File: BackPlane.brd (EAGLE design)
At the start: 134.6 x 116.5 mm, 1 part

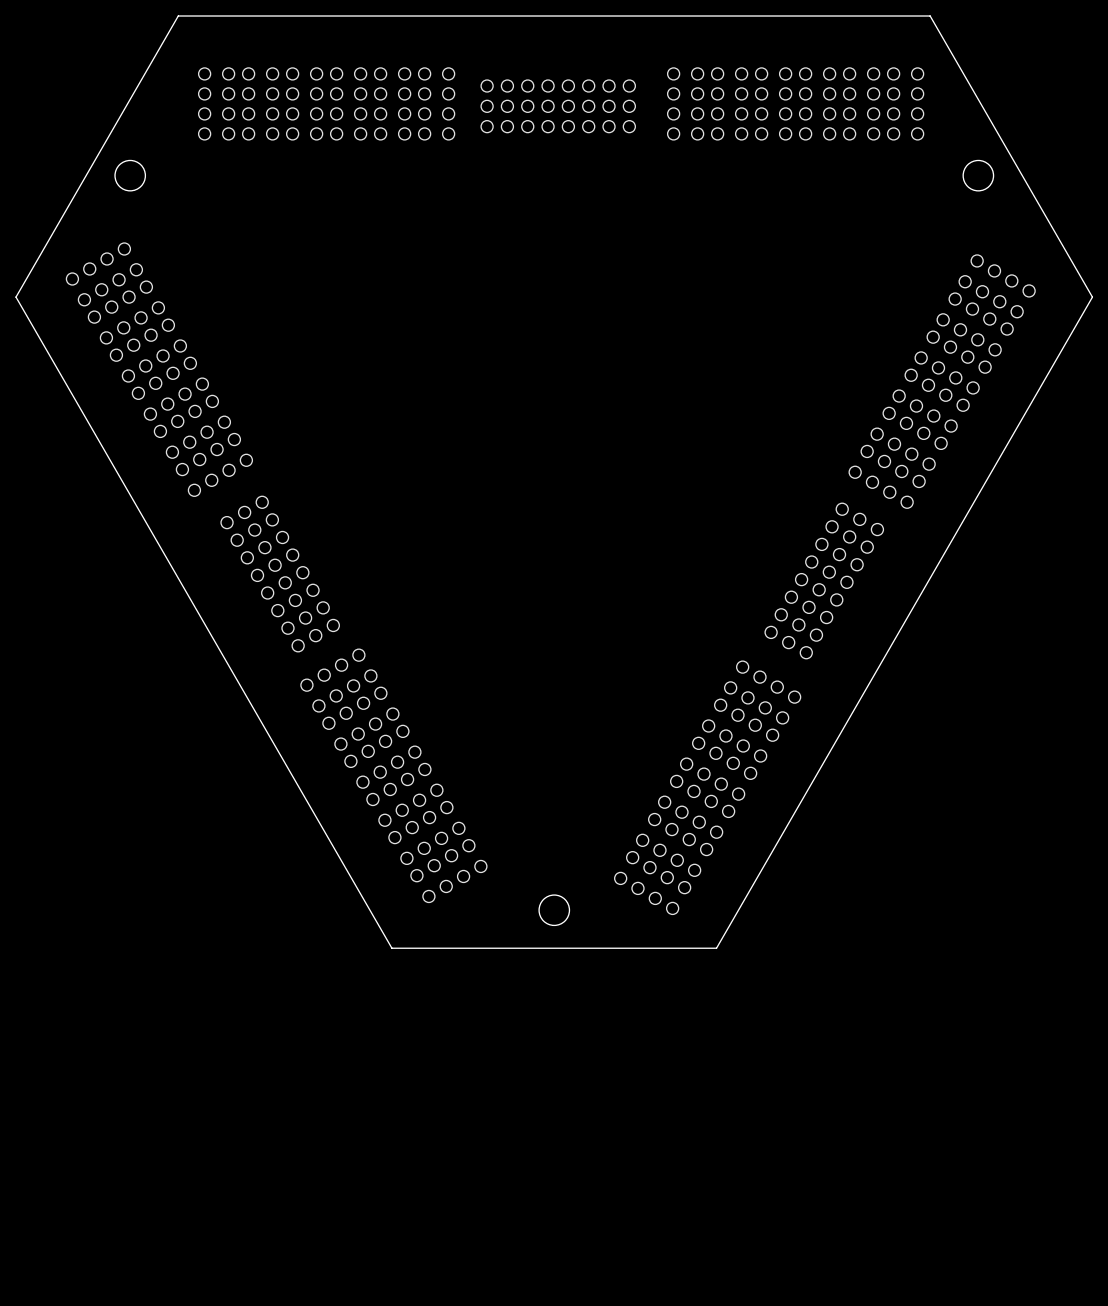
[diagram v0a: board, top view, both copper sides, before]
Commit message: progress
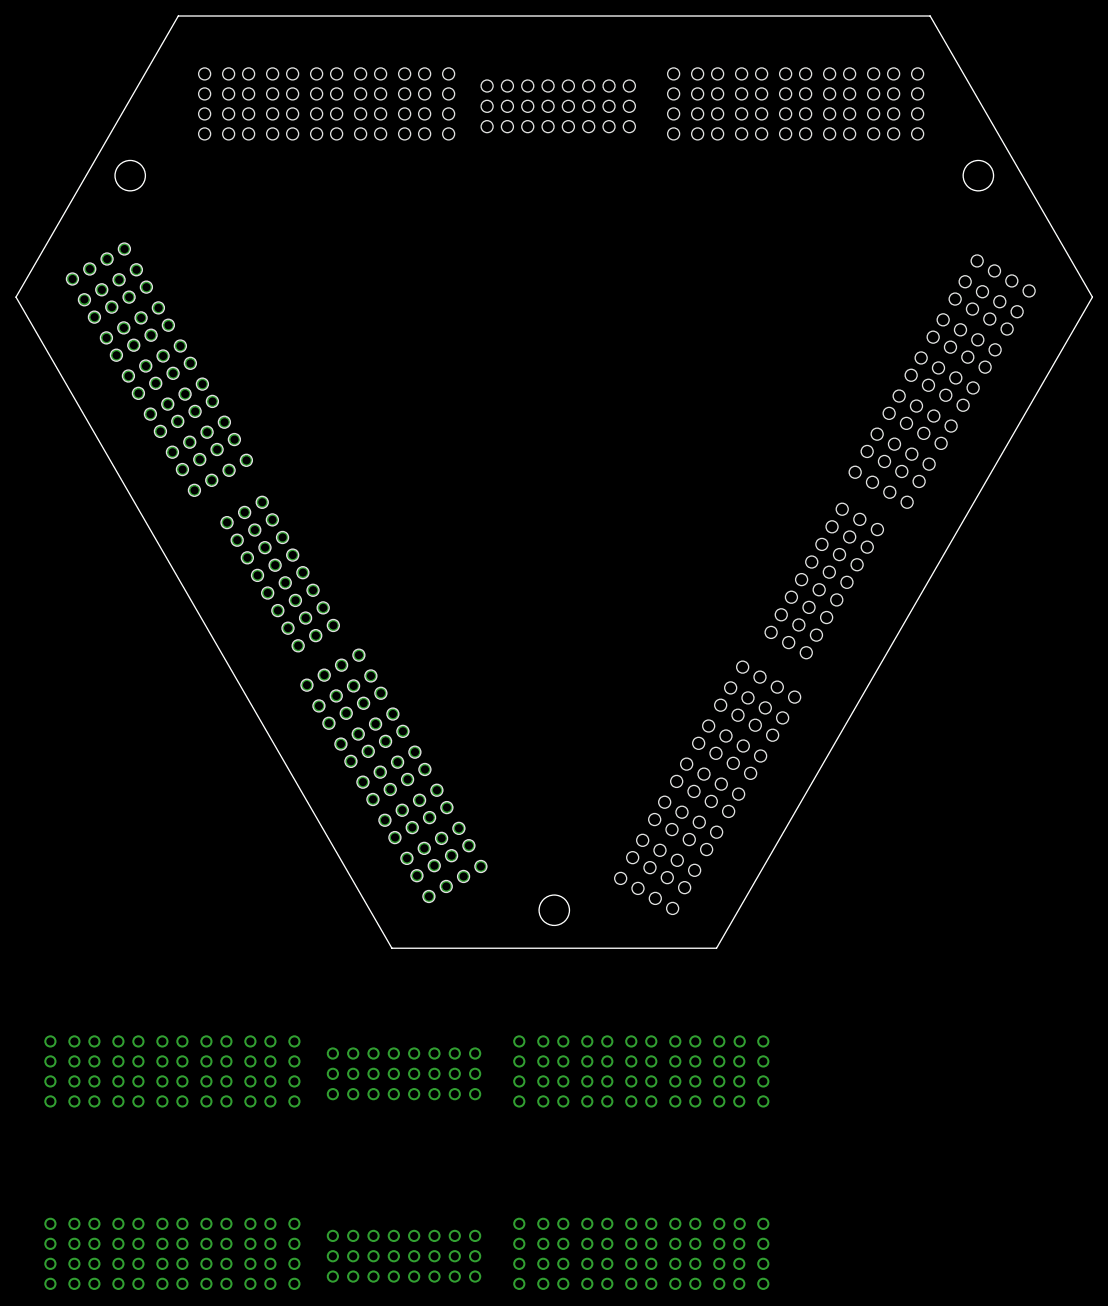
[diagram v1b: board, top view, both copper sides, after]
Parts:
- added U$2, U$3, U$4: THICC_CONNECTOR, THICC_CONNECTOR:THICC_CONNECTOR
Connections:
- new net +12V: U$2.15, U$2.16, U$2.23, U$2.24, U$3.15, U$3.16, U$3.23, U$3.24, U$4.15, U$4.16, U$4.23, U$4.24
- new net +12V_GND: U$2.13, U$2.14, U$2.21, U$2.22, U$3.13, U$3.14, U$3.21, U$3.22, U$4.13, U$4.14, U$4.21, U$4.22
- new net +5V: U$2.11, U$2.12, U$2.19, U$2.20, U$3.11, U$3.12, U$3.19, U$3.20, U$4.11, U$4.12, U$4.19, U$4.20
- new net +5V_GND: U$2.10, U$2.17, U$2.18, U$2.9, U$3.10, U$3.17, U$3.18, U$3.9, U$4.10, U$4.17, U$4.18, U$4.9
- new net B1: U$2.P1-13, U$2.P1-14, U$2.P1-15, U$2.P1-16, U$2.P2-17, U$2.P2-18, U$2.P2-19, U$2.P2-20, U$4.P1-13, U$4.P1-14, U$4.P1-15, U$4.P1-16, U$4.P2-17, U$4.P2-18, U$4.P2-19, U$4.P2-20
- new net B2: U$2.P2-1, U$2.P2-2, U$2.P2-3, U$2.P2-4, U$2.P2-5, U$2.P2-6, U$2.P2-7, U$2.P2-8, U$4.P2-1, U$4.P2-2, U$4.P2-3, U$4.P2-4, U$4.P2-5, U$4.P2-6, U$4.P2-7, U$4.P2-8
- new net B3: U$2.P3-25, U$2.P3-26, U$2.P3-27, U$2.P3-28, U$2.P4-5, U$2.P4-6, U$2.P4-7, U$2.P4-8, U$3.P3-25, U$3.P3-26, U$3.P3-27, U$3.P3-28, U$3.P4-5, U$3.P4-6, U$3.P4-7, U$3.P4-8, U$4.P3-25, U$4.P3-26, U$4.P3-27, U$4.P3-28, U$4.P4-5, U$4.P4-6, U$4.P4-7, U$4.P4-8
- new net B4: U$2.P3-13, U$2.P3-14, U$2.P3-15, U$2.P3-16, U$2.P4-10, U$2.P4-11, U$2.P4-12, U$2.P4-9, U$3.P3-13, U$3.P3-14, U$3.P3-15, U$3.P3-16, U$3.P4-10, U$3.P4-11, U$3.P4-12, U$3.P4-9, U$4.P3-13, U$4.P3-14, U$4.P3-15, U$4.P3-16, U$4.P4-10, U$4.P4-11, U$4.P4-12, U$4.P4-9
- new net B5: U$3.P1-13, U$3.P1-14, U$3.P1-15, U$3.P1-16, U$3.P2-17, U$3.P2-18, U$3.P2-19, U$3.P2-20
- new net B6: U$3.P2-1, U$3.P2-2, U$3.P2-3, U$3.P2-4, U$3.P2-5, U$3.P2-6, U$3.P2-7, U$3.P2-8
- new net CAN_H: U$2.8, U$3.8, U$4.8
- new net CAN_L: U$2.7, U$3.7, U$4.7
- new net R1: U$2.P1-1, U$2.P1-2, U$2.P1-21, U$2.P1-22, U$2.P1-23, U$2.P1-24, U$2.P1-3, U$2.P1-4, U$4.P1-1, U$4.P1-2, U$4.P1-21, U$4.P1-22, U$4.P1-23, U$4.P1-24, U$4.P1-3, U$4.P1-4
- new net R2: U$2.P1-10, U$2.P1-11, U$2.P1-12, U$2.P1-9, U$2.P2-13, U$2.P2-14, U$2.P2-15, U$2.P2-16, U$4.P1-10, U$4.P1-11, U$4.P1-12, U$4.P1-9, U$4.P2-13, U$4.P2-14, U$4.P2-15, U$4.P2-16
- new net R3: U$2.P3-17, U$2.P3-18, U$2.P3-19, U$2.P3-20, U$2.P4-13, U$2.P4-14, U$2.P4-15, U$2.P4-16, U$3.P3-17, U$3.P3-18, U$3.P3-19, U$3.P3-20, U$4.P3-17, U$4.P3-18, U$4.P3-19, U$4.P3-20, U$4.P4-13, U$4.P4-14, U$4.P4-15, U$4.P4-16
- new net R4: U$2.P3-1, U$2.P3-2, U$2.P3-3, U$2.P3-4, U$2.P3-5, U$2.P3-6, U$2.P3-7, U$2.P3-8, U$3.P3-1, U$3.P3-2, U$3.P3-3, U$3.P3-4, U$3.P3-5, U$3.P3-6, U$3.P3-7, U$3.P3-8, U$4.P3-1, U$4.P3-2, U$4.P3-3, U$4.P3-4, U$4.P3-5, U$4.P3-6, U$4.P3-7, U$4.P3-8
- new net R5: U$3.P1-1, U$3.P1-2, U$3.P1-21, U$3.P1-22, U$3.P1-23, U$3.P1-24, U$3.P1-3, U$3.P1-4
- new net R6: U$3.P1-10, U$3.P1-11, U$3.P1-12, U$3.P1-9, U$3.P2-13, U$3.P2-14, U$3.P2-15, U$3.P2-16
- new net R7: U$3.P4-13, U$3.P4-14, U$3.P4-15, U$3.P4-16
- new net Y1: U$2.P1-17, U$2.P1-18, U$2.P1-19, U$2.P1-20, U$2.P2-21, U$2.P2-22, U$2.P2-23, U$2.P2-24, U$4.P1-17, U$4.P1-18, U$4.P1-19, U$4.P1-20, U$4.P2-21, U$4.P2-22, U$4.P2-23, U$4.P2-24
- new net Y2: U$2.P1-5, U$2.P1-6, U$2.P1-7, U$2.P1-8, U$2.P2-10, U$2.P2-11, U$2.P2-12, U$2.P2-9, U$4.P1-5, U$4.P1-6, U$4.P1-7, U$4.P1-8, U$4.P2-10, U$4.P2-11, U$4.P2-12, U$4.P2-9
- new net Y3: U$2.P4-17, U$2.P4-18, U$2.P4-19, U$2.P4-20, U$2.P4-25, U$2.P4-26, U$2.P4-27, U$2.P4-28, U$4.P4-17, U$4.P4-18, U$4.P4-19, U$4.P4-20, U$4.P4-25, U$4.P4-26, U$4.P4-27, U$4.P4-28
- new net Y4: U$2.P3-10, U$2.P3-11, U$2.P3-12, U$2.P3-9, U$2.P4-1, U$2.P4-2, U$2.P4-3, U$2.P4-4, U$3.P3-10, U$3.P3-11, U$3.P3-12, U$3.P3-9, U$3.P4-1, U$3.P4-2, U$3.P4-3, U$3.P4-4, U$4.P3-10, U$4.P3-11, U$4.P3-12, U$4.P3-9, U$4.P4-1, U$4.P4-2, U$4.P4-3, U$4.P4-4
- new net Y5: U$3.P1-17, U$3.P1-18, U$3.P1-19, U$3.P1-20, U$3.P2-21, U$3.P2-22, U$3.P2-23, U$3.P2-24
- new net Y6: U$3.P1-5, U$3.P1-6, U$3.P1-7, U$3.P1-8, U$3.P2-10, U$3.P2-11, U$3.P2-12, U$3.P2-9
- new net Y7: U$3.P4-17, U$3.P4-18, U$3.P4-19, U$3.P4-20, U$3.P4-25, U$3.P4-26, U$3.P4-27, U$3.P4-28

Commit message: names
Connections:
- new net B10: U$4.P2-1, U$4.P2-2, U$4.P2-3, U$4.P2-4, U$4.P2-5, U$4.P2-6, U$4.P2-7, U$4.P2-8
- new net B11: U$4.P3-25, U$4.P3-26, U$4.P3-27, U$4.P3-28, U$4.P4-5, U$4.P4-6, U$4.P4-7, U$4.P4-8
- new net B12: U$4.P3-13, U$4.P3-14, U$4.P3-15, U$4.P3-16, U$4.P4-10, U$4.P4-11, U$4.P4-12, U$4.P4-9
- new net B7: U$3.P4-5, U$3.P4-6, U$3.P4-7, U$3.P4-8
- new net B8: U$3.P3-13, U$3.P3-14, U$3.P3-15, U$3.P3-16, U$3.P4-10, U$3.P4-11, U$3.P4-12, U$3.P4-9
- new net B9: U$4.P1-13, U$4.P1-14, U$4.P1-15, U$4.P1-16, U$4.P2-17, U$4.P2-18, U$4.P2-19, U$4.P2-20
- new net BY: U$3.P3-25, U$3.P3-26, U$3.P3-27, U$3.P3-28
- new net R10: U$4.P1-10, U$4.P1-11, U$4.P1-12, U$4.P1-9, U$4.P2-13, U$4.P2-14, U$4.P2-15, U$4.P2-16
- new net R11: U$4.P3-17, U$4.P3-18, U$4.P3-19, U$4.P3-20, U$4.P4-13, U$4.P4-14, U$4.P4-15, U$4.P4-16
- new net R12: U$4.P3-1, U$4.P3-2, U$4.P3-3, U$4.P3-4, U$4.P3-5, U$4.P3-6, U$4.P3-7, U$4.P3-8
- new net R8: U$3.P3-1, U$3.P3-2, U$3.P3-3, U$3.P3-4, U$3.P3-5, U$3.P3-6, U$3.P3-7, U$3.P3-8
- new net R9: U$4.P1-1, U$4.P1-2, U$4.P1-21, U$4.P1-22, U$4.P1-23, U$4.P1-24, U$4.P1-3, U$4.P1-4
- new net Y10: U$4.P1-5, U$4.P1-6, U$4.P1-7, U$4.P1-8, U$4.P2-10, U$4.P2-11, U$4.P2-12, U$4.P2-9
- new net Y11: U$4.P4-17, U$4.P4-18, U$4.P4-19, U$4.P4-20, U$4.P4-25, U$4.P4-26, U$4.P4-27, U$4.P4-28
- new net Y12: U$4.P3-10, U$4.P3-11, U$4.P3-12, U$4.P3-9, U$4.P4-1, U$4.P4-2, U$4.P4-3, U$4.P4-4
- new net Y8: U$3.P3-10, U$3.P3-11, U$3.P3-12, U$3.P3-9, U$3.P4-1, U$3.P4-2, U$3.P4-3, U$3.P4-4
- new net Y9: U$4.P1-17, U$4.P1-18, U$4.P1-19, U$4.P1-20, U$4.P2-21, U$4.P2-22, U$4.P2-23, U$4.P2-24
- net B1: no longer U$4.P1-13, U$4.P1-14, U$4.P1-15, U$4.P1-16, U$4.P2-17, U$4.P2-18, U$4.P2-19, U$4.P2-20
- net B2: no longer U$4.P2-1, U$4.P2-2, U$4.P2-3, U$4.P2-4, U$4.P2-5, U$4.P2-6, U$4.P2-7, U$4.P2-8
- net B3: no longer U$3.P3-25, U$3.P3-26, U$3.P3-27, U$3.P3-28, U$3.P4-5, U$3.P4-6, U$3.P4-7, U$3.P4-8, U$4.P3-25, U$4.P3-26, U$4.P3-27, U$4.P3-28, U$4.P4-5, U$4.P4-6, U$4.P4-7, U$4.P4-8
- net B4: no longer U$3.P3-13, U$3.P3-14, U$3.P3-15, U$3.P3-16, U$3.P4-10, U$3.P4-11, U$3.P4-12, U$3.P4-9, U$4.P3-13, U$4.P3-14, U$4.P3-15, U$4.P3-16, U$4.P4-10, U$4.P4-11, U$4.P4-12, U$4.P4-9
- net R1: no longer U$4.P1-1, U$4.P1-2, U$4.P1-21, U$4.P1-22, U$4.P1-23, U$4.P1-24, U$4.P1-3, U$4.P1-4
- net R2: no longer U$4.P1-10, U$4.P1-11, U$4.P1-12, U$4.P1-9, U$4.P2-13, U$4.P2-14, U$4.P2-15, U$4.P2-16
- net R3: no longer U$3.P3-17, U$3.P3-18, U$3.P3-19, U$3.P3-20, U$4.P3-17, U$4.P3-18, U$4.P3-19, U$4.P3-20, U$4.P4-13, U$4.P4-14, U$4.P4-15, U$4.P4-16
- net R4: no longer U$3.P3-1, U$3.P3-2, U$3.P3-3, U$3.P3-4, U$3.P3-5, U$3.P3-6, U$3.P3-7, U$3.P3-8, U$4.P3-1, U$4.P3-2, U$4.P3-3, U$4.P3-4, U$4.P3-5, U$4.P3-6, U$4.P3-7, U$4.P3-8
- net R7: now also U$3.P3-17, U$3.P3-18, U$3.P3-19, U$3.P3-20
- net Y1: no longer U$4.P1-17, U$4.P1-18, U$4.P1-19, U$4.P1-20, U$4.P2-21, U$4.P2-22, U$4.P2-23, U$4.P2-24
- net Y2: no longer U$4.P1-5, U$4.P1-6, U$4.P1-7, U$4.P1-8, U$4.P2-10, U$4.P2-11, U$4.P2-12, U$4.P2-9
- net Y3: no longer U$4.P4-17, U$4.P4-18, U$4.P4-19, U$4.P4-20, U$4.P4-25, U$4.P4-26, U$4.P4-27, U$4.P4-28
- net Y4: no longer U$3.P3-10, U$3.P3-11, U$3.P3-12, U$3.P3-9, U$3.P4-1, U$3.P4-2, U$3.P4-3, U$3.P4-4, U$4.P3-10, U$4.P3-11, U$4.P3-12, U$4.P3-9, U$4.P4-1, U$4.P4-2, U$4.P4-3, U$4.P4-4
